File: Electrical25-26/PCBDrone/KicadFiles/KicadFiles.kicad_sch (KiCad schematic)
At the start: 17 parts, among them J1 Conn_01x02_Pin, U1 ESP32-WROOM-32E, U2 BMI323, U3 DRV8210DSGR

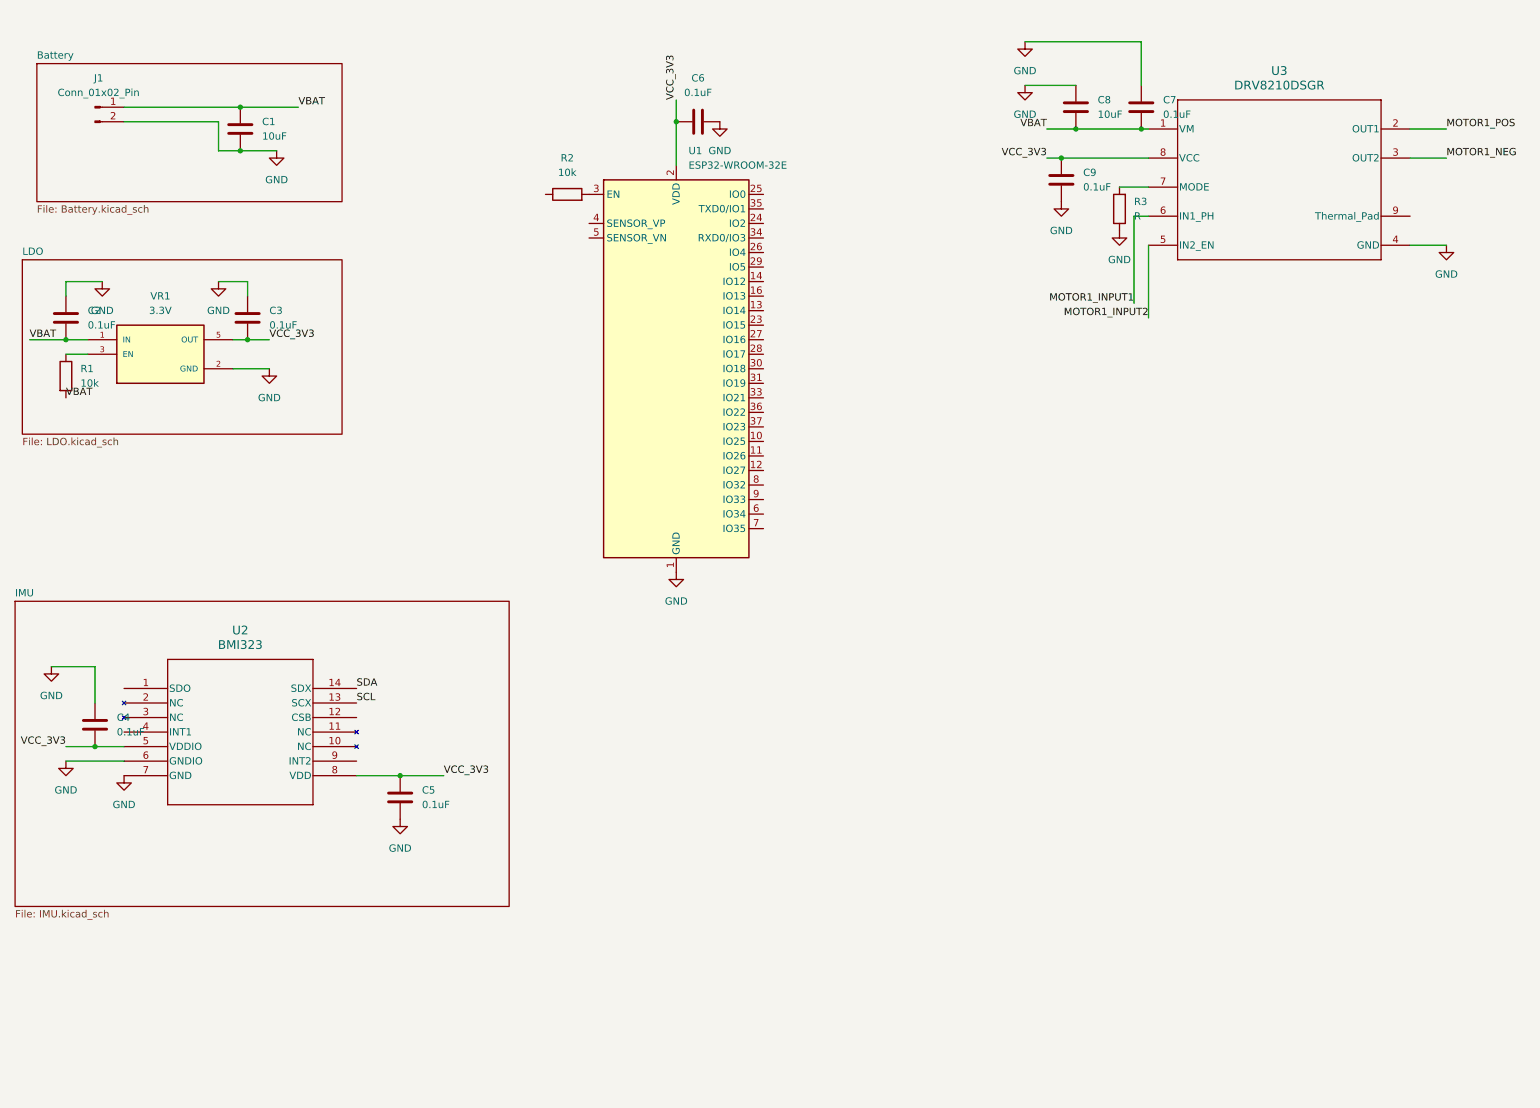
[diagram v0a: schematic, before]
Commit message: Schematic tentatively done
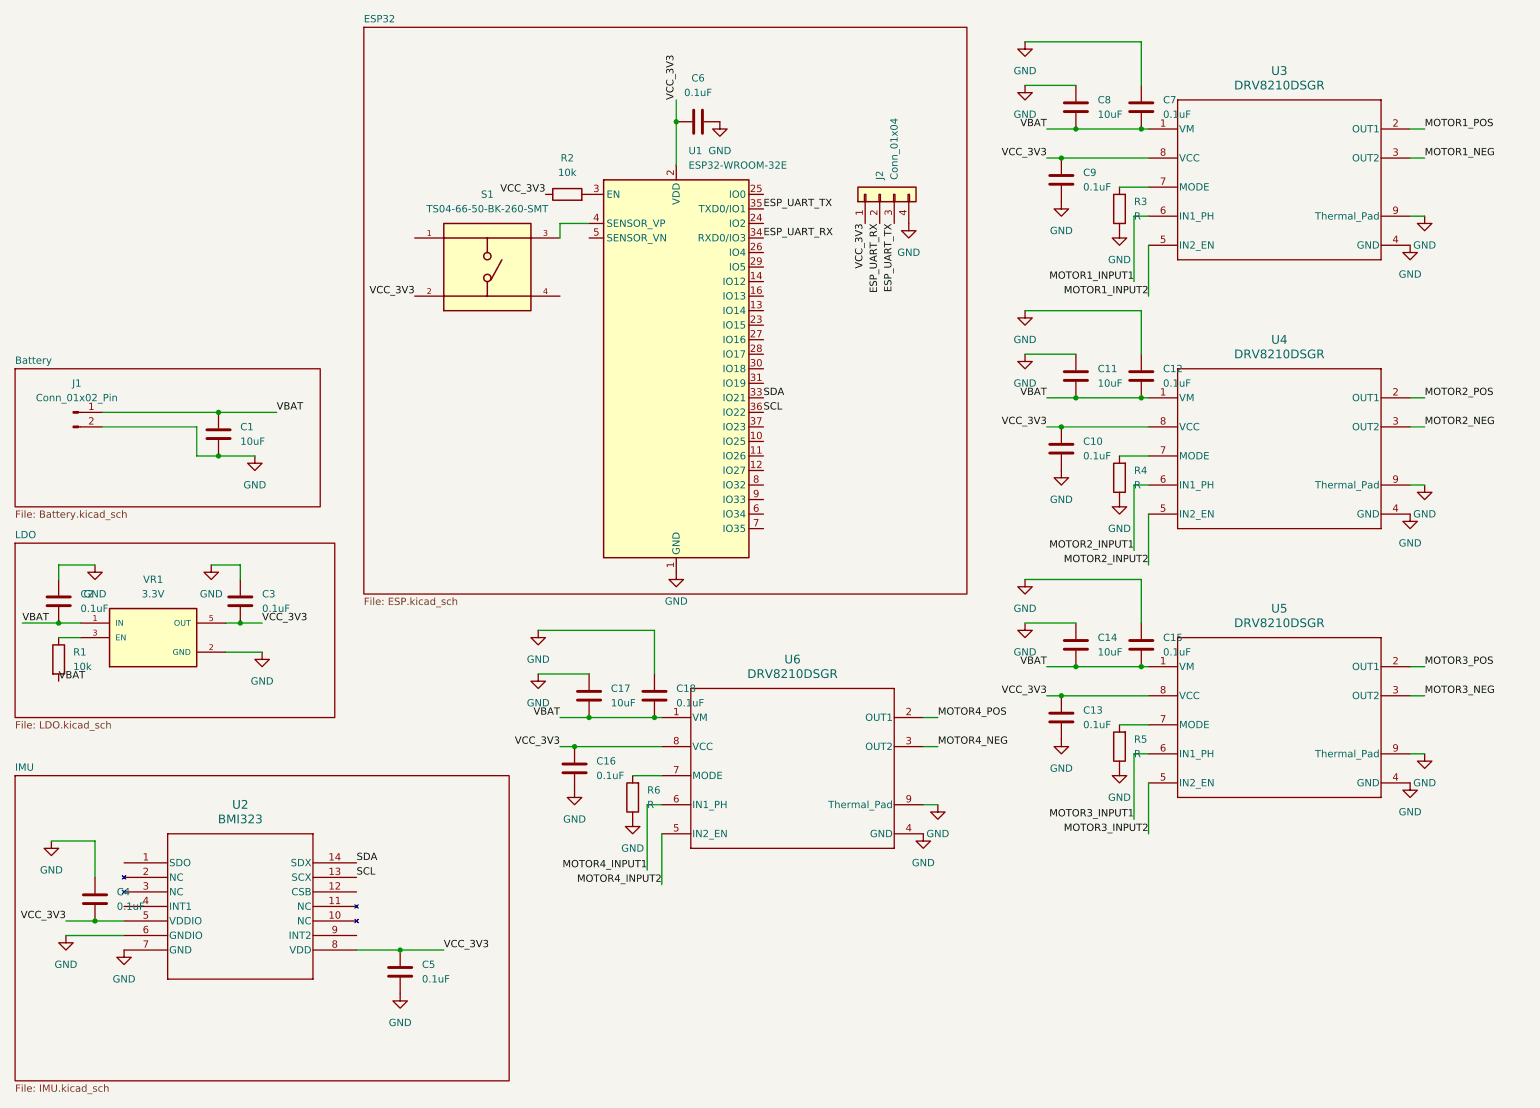
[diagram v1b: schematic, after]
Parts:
- added C10, C12, C13, C15, C16, C18: 0.1uF, symbol Device:C
- added C11, C14, C17: 10uF, symbol Device:C
- added J2: Conn_01x04, symbol Connector_Generic:Conn_01x04
- added R4, R5, R6: R, symbol Device:R
- added S1: TS04-66-50-BK-260-SMT, TS04-66-50-BK-260-SMT:SW_TS04-66-50-BK-260-SMT, symbol TS04-66-50-BK-260-SMT:TS04-66-50-BK-260-SMT
- added U4, U5, U6: DRV8210DSGR, DSG0008A-IPC_A, symbol 2025-09-15_20-21-28:DRV8210DSGR
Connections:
- net GND: now also U3.9 (Thermal_Pad), C10.2, C11.1, C12.1, C13.2, C14.1, C15.1, C16.2, C17.1, C18.1, J2.4 (Pin_4), R4.1, R5.1, R6.1, U4.4 (GND), U4.9 (Thermal_Pad), U5.4 (GND), U5.9 (Thermal_Pad), U6.4 (GND), U6.9 (Thermal_Pad)
- net SCL: now also U1.36 (IO22)
- net SDA: now also U1.33 (IO21)
- net VBAT: now also C11.2, C12.2, C14.2, C15.2, C17.2, C18.2, U4.1 (VM), U5.1 (VM), U6.1 (VM)
- net VCC_3V3: now also R2.1, C10.1, C13.1, C16.1, J2.1 (Pin_1), S1.2, U4.8 (VCC), U5.8 (VCC), U6.8 (VCC)
- net ESP_UART_RX: now reaches U1.34 (RXD0/IO3)
- net ESP_UART_RX: now also J2.2 (Pin_2)
- net ESP_UART_TX: now reaches U1.35 (TXD0/IO1)
- net ESP_UART_TX: now also J2.3 (Pin_3)
- net at U1.4 (SENSOR_VP): now also S1.3
- new net: R6.2, U6.7 (MODE)
- new net: R4.2, U4.7 (MODE)
- new net: R5.2, U5.7 (MODE)
- new net MOTOR2_INPUT1: U4.6 (IN1_PH)
- new net MOTOR2_INPUT2: U4.5 (IN2_EN)
- new net MOTOR2_NEG: U4.3 (OUT2)
- new net MOTOR2_POS: U4.2 (OUT1)
- new net MOTOR3_INPUT1: U5.6 (IN1_PH)
- new net MOTOR3_INPUT2: U5.5 (IN2_EN)
- new net MOTOR3_NEG: U5.3 (OUT2)
- new net MOTOR3_POS: U5.2 (OUT1)
- new net MOTOR4_INPUT1: U6.6 (IN1_PH)
- new net MOTOR4_INPUT2: U6.5 (IN2_EN)
- new net MOTOR4_NEG: U6.3 (OUT2)
- new net MOTOR4_POS: U6.2 (OUT1)
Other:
- added sheet ESP32 (ESP.kicad_sch)
- moved on the sheet: C1, C2, C3, C4, C5, J1, R1, U2, VR1
